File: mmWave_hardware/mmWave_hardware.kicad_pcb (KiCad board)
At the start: 6 copper layers, 49 x 21.6 mm, 48 parts, among them J1 Conn_02x08_Top_Bottom, U1 IWRL6432BDBAAMFR, U2 W25Q128JVS, U3 AMS1117-3.3, U4 TPS628502QDRLRQ1, Y1 40.000

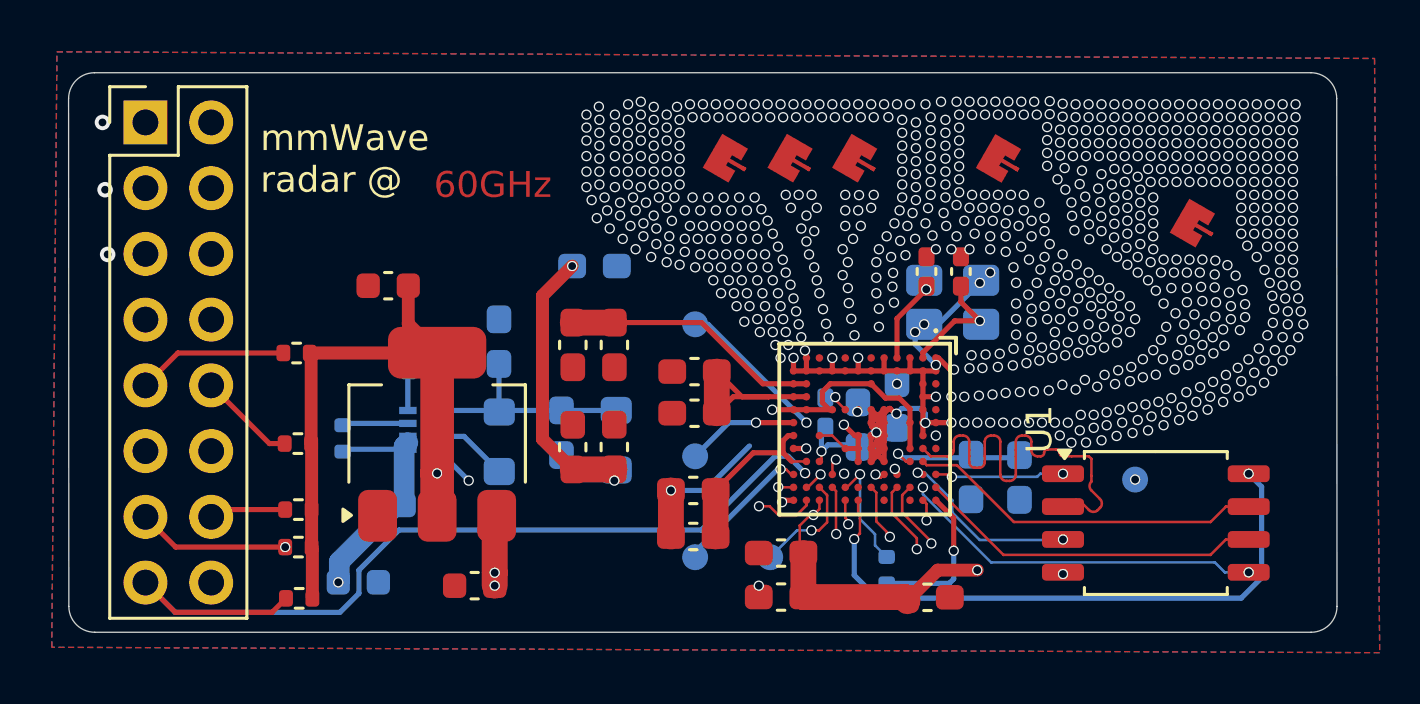
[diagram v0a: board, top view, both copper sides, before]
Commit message: unrouted all
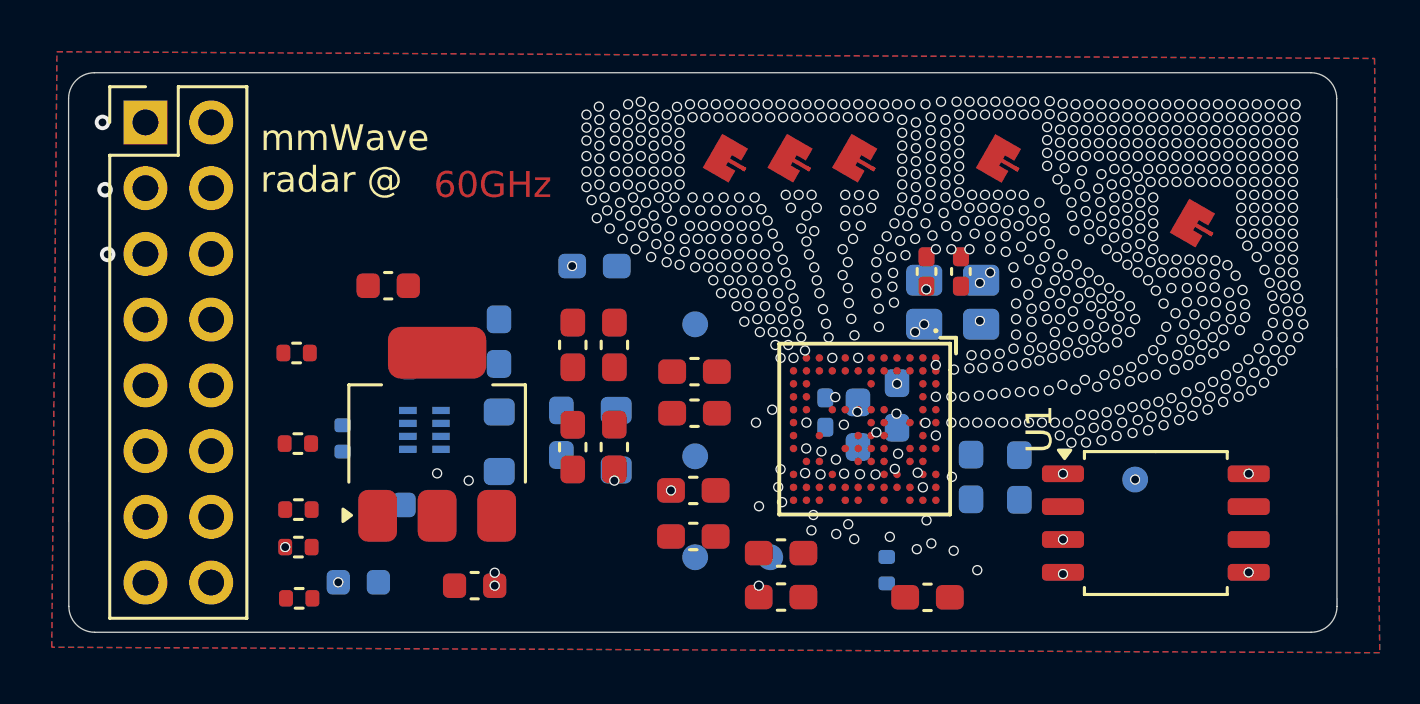
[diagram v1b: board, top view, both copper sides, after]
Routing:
- net GND: track 75.7 -> 0.00 mm
- net 1v8: track 70.7 -> 0.00 mm
- net 3v3: track 66.2 -> 0.00 mm
- net RS232_TX: track 52.1 -> 0.00 mm
- net SPI0_CLK: track 51.7 -> 0.00 mm
- net RS232_RX: track 51.0 -> 0.00 mm
- net SPI0_CS0_N: track 48.9 -> 0.00 mm
- net SPI0_MISO: track 45.0 -> 0.00 mm
- net SPI0_MOSI: track 44.9 -> 0.00 mm
- net UART_RX: track 40.4 -> 0.00 mm
- net GPIO_2: track 39.0 -> 0.00 mm
- net UART_TX: track 36.8 -> 0.00 mm
- net NRST_MAIN: track 35.4 -> 0.00 mm
- net VIN: track 23.0 -> 0.00 mm
- net /QSPI_1: track 17.1 -> 0.00 mm
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
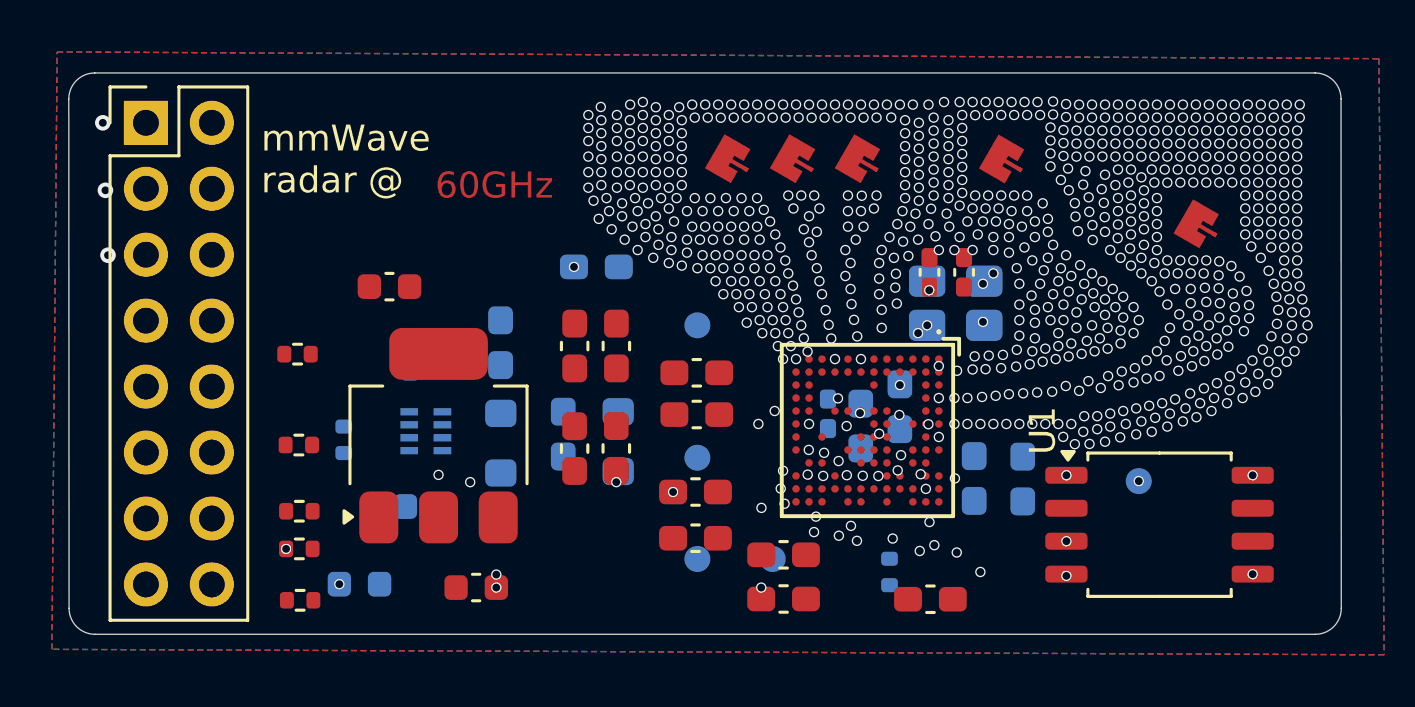
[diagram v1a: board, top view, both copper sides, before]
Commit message: routing done
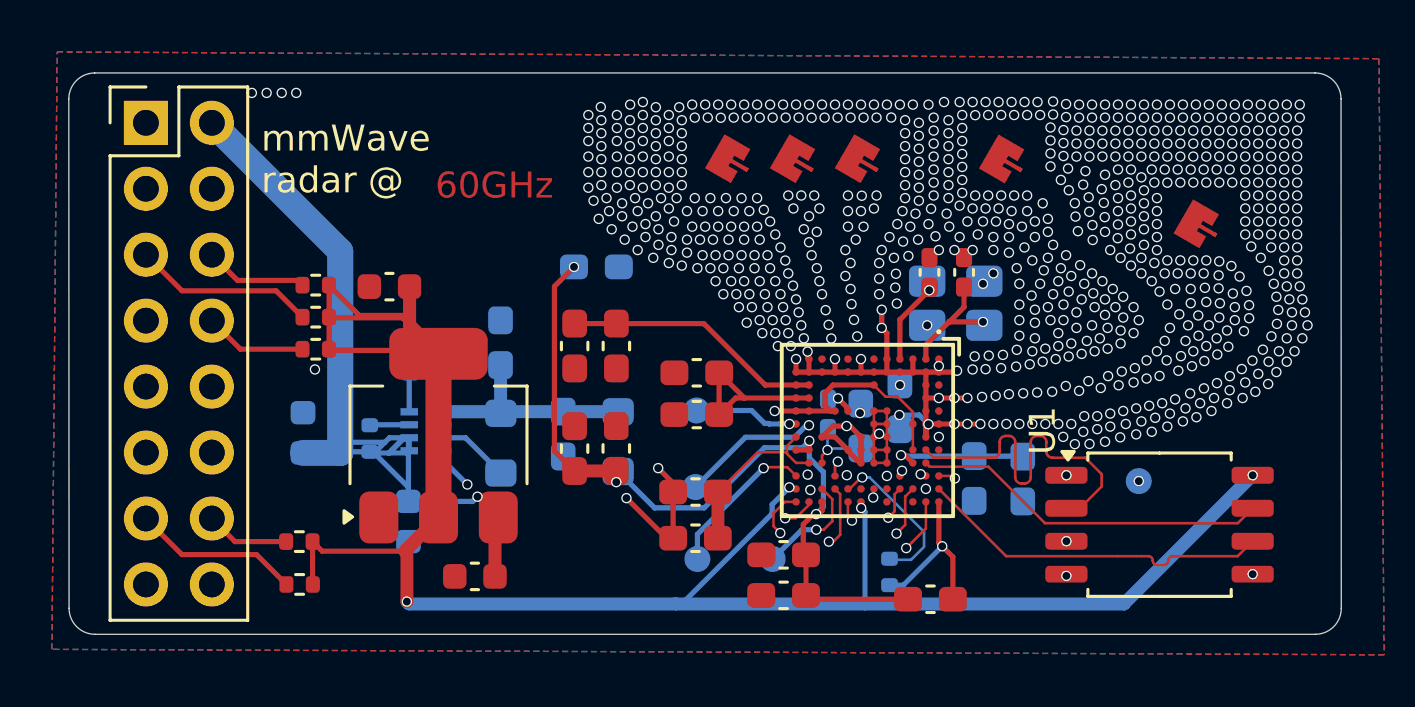
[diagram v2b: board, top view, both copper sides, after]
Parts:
- moved R3 10.2 mm to (58.5, 61.6)
- moved R6 9.69 mm to (58.5, 64.0)
- moved R2 7.50 mm to (58.5, 62.8)
- moved R4 7.22 mm to (57.9, 71.4)
- moved TP5 6.23 mm to (73.1, 69.3)
- moved C20 6.22 mm to (58.0, 67.2), turned to 90 degrees
- moved R5 5.37 mm to (57.9, 73.1)
- moved TP4 1.82 mm to (73.2, 66.4)
- moved R7 1.00 mm to (60.6, 67.5)
- moved C21 0.88 mm to (62.1, 70.7), turned to -90 degrees
- moved C18 0.43 mm to (64.6, 72.8)
- moved C9 0.14 mm to (76.5, 73.5)
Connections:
- J1 pad 10: SPI0_CS0_N -> UART_RTS
- J1 pad 11: SPI0_MISO -> UART_RX
- J1 pad 12: SPI0_MOSI -> UART_TX
- J1 pad 13: RS232_TX -> SPI0_CS0_N
- J1 pad 14: RS232_RX -> SPI0_CLK
- J1 pad 15: NRST_MAIN -> SPI0_MOSI
- J1 pad 16: VIN -> SPI0_MISO
- J1 pad 2: GPIO_2 -> VIN
- J1 pad 3: GND -> GPIO_2
- J1 pad 5: GND -> RS232_RX
- J1 pad 6: UART_RTS -> RS232_TX
- J1 pad 7: UART_RX -> unconnected-(J1-Pin_7-Pad7)
- J1 pad 8: UART_TX -> NRST_MAIN
- J1 pad 9: SPI0_CLK -> unconnected-(J1-Pin_9-Pad9)
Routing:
- net 3v3: track 0.00 -> 80.6 mm
- net GND: track 0.00 -> 52.3 mm
- net SPI0_CS0_N: track 0.00 -> 42.8 mm
- net 1v8: track 0.00 -> 42.5 mm, vias 6 -> 5
- net RS232_RX: track 0.00 -> 38.9 mm
- net SPI0_CLK: track 0.00 -> 38.0 mm
- net VIN: track 0.00 -> 35.1 mm, vias 3 -> 1
- net RS232_TX: track 0.00 -> 35.0 mm, vias 2 -> 1
- net SPI0_MOSI: track 0.00 -> 33.7 mm
- net SPI0_MISO: track 0.00 -> 33.7 mm
- net GPIO_2: track 0.00 -> 31.7 mm
- net UART_RX: track 0.00 -> 30.3 mm
- net UART_TX: track 0.00 -> 30.1 mm
- net NRST_MAIN: track 0.00 -> 29.6 mm
- net GPIO_5: track 0.00 -> 29.1 mm
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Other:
- board text removed: "ABCS"
- board text removed: "If you can see this, You have voided your warranty"

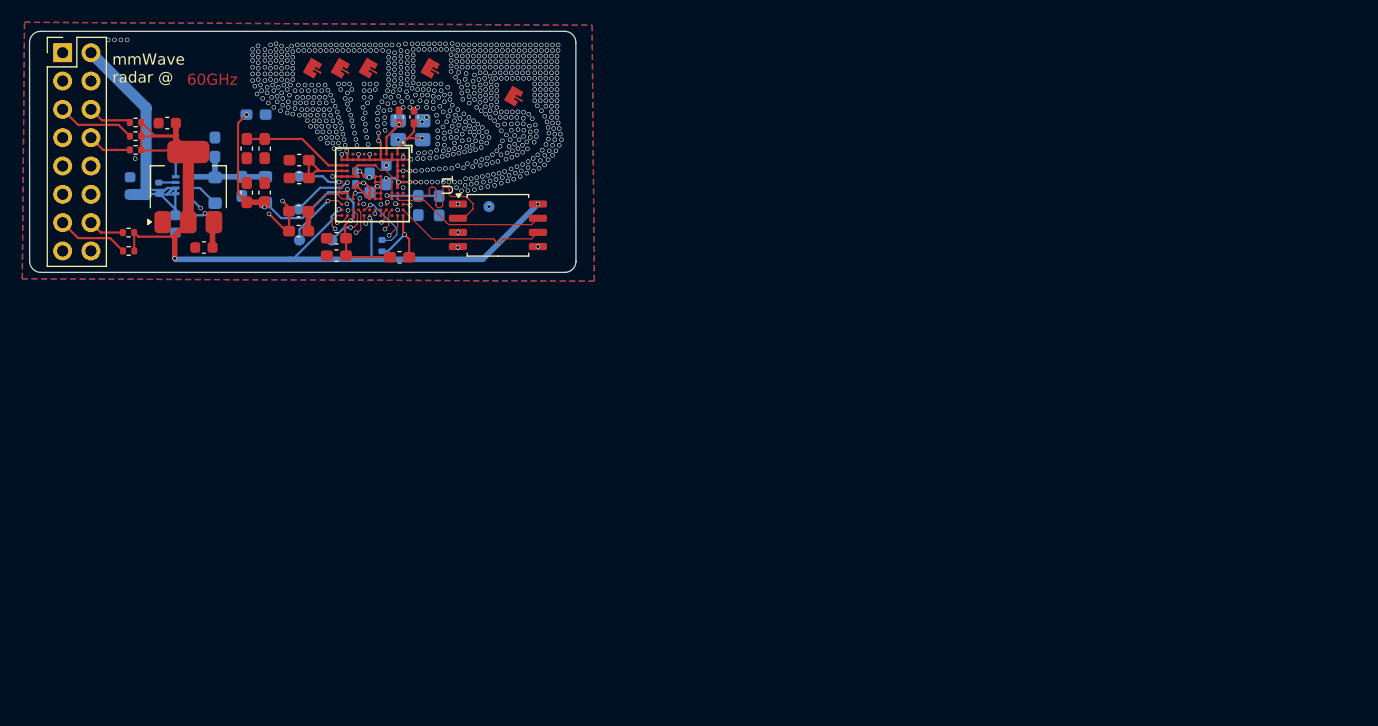
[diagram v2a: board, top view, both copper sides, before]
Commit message: Final PCB(Probably)
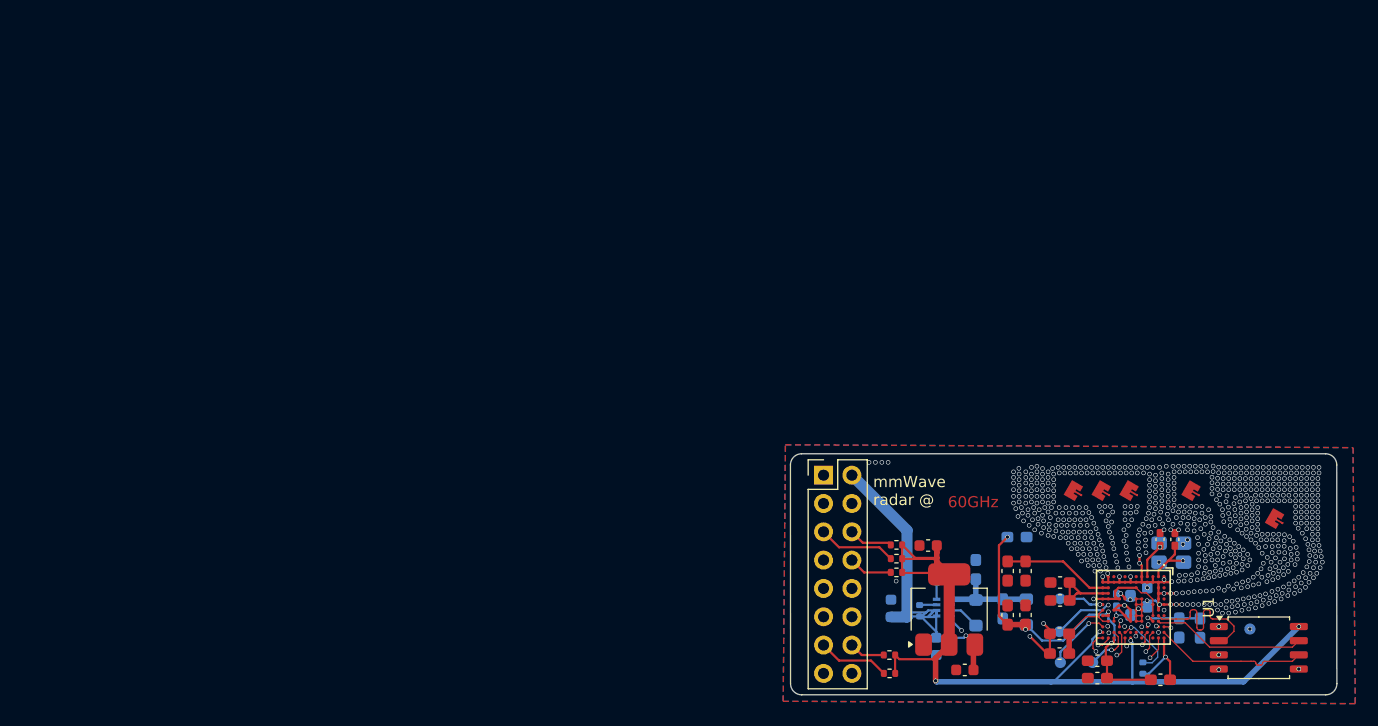
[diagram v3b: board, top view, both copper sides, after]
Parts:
- moved C10 78.1 mm to (144.8, 109.8)
- moved C11 78.1 mm to (141.4, 107.4)
- moved C12 78.1 mm to (141.4, 109.2)
- moved C13 78.1 mm to (136.7, 105.7)
- moved C14 78.1 mm to (138.3, 105.7)
- moved C17 78.1 mm to (149.2, 104.1)
- moved C18 78.1 mm to (132.9, 110.7)
- moved C19 78.1 mm to (129.6, 99.5)
- moved C2 78.1 mm to (151.7, 99.0)
- moved C20 78.1 mm to (126.3, 105.1)
- moved C21 78.1 mm to (130.3, 108.5)
- moved C22 78.1 mm to (136.3, 105.2)
- moved C23 78.1 mm to (137.6, 98.7)
- moved C24 78.1 mm to (133.9, 101.7)
- moved C3 78.1 mm to (152.1, 106.9)
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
